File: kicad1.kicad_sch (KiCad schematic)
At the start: 44 parts

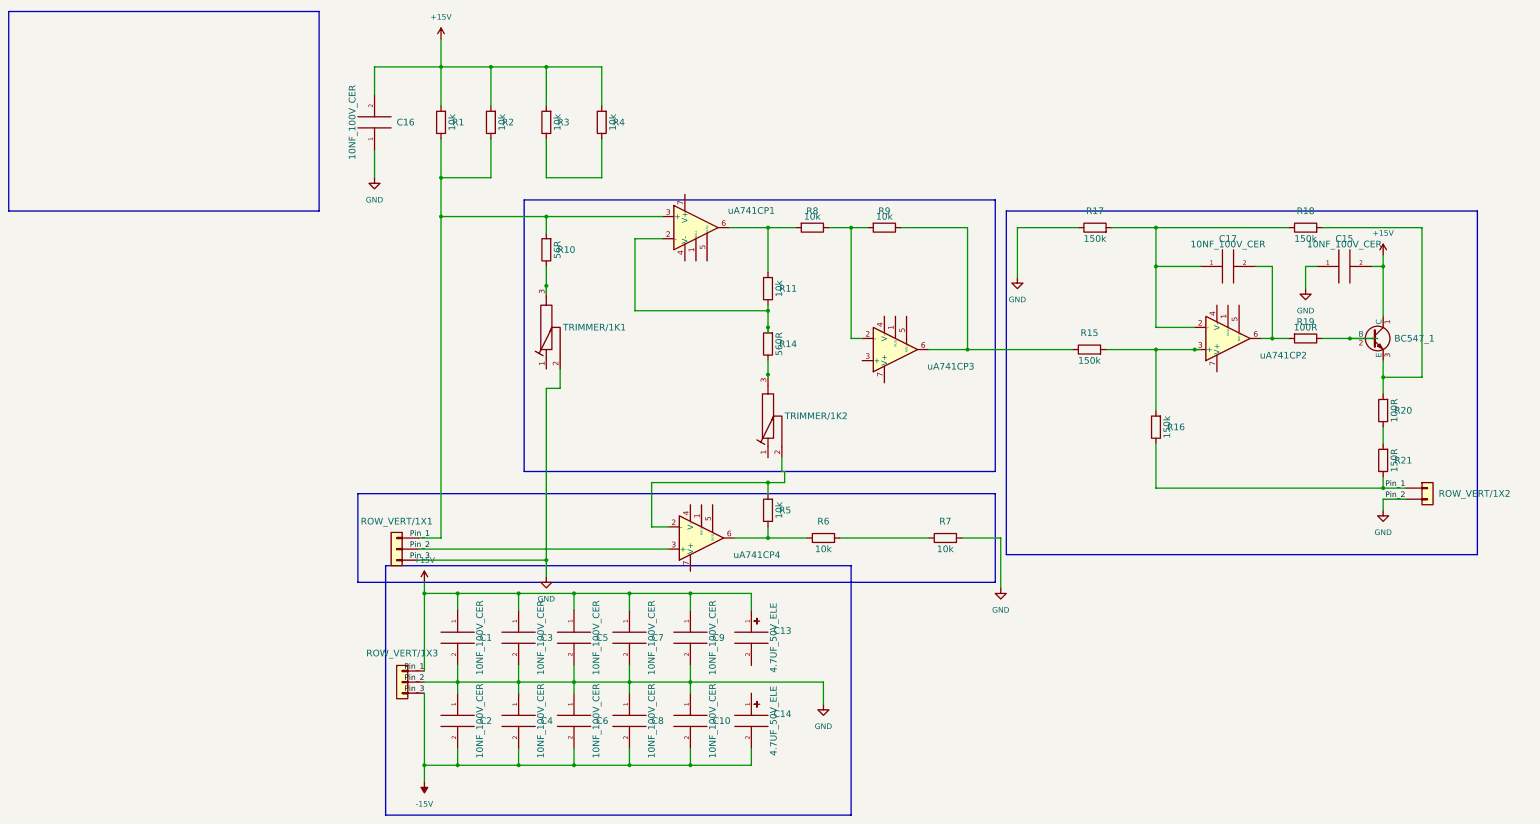
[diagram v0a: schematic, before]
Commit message: epätoivoinen versio ennen resettiä
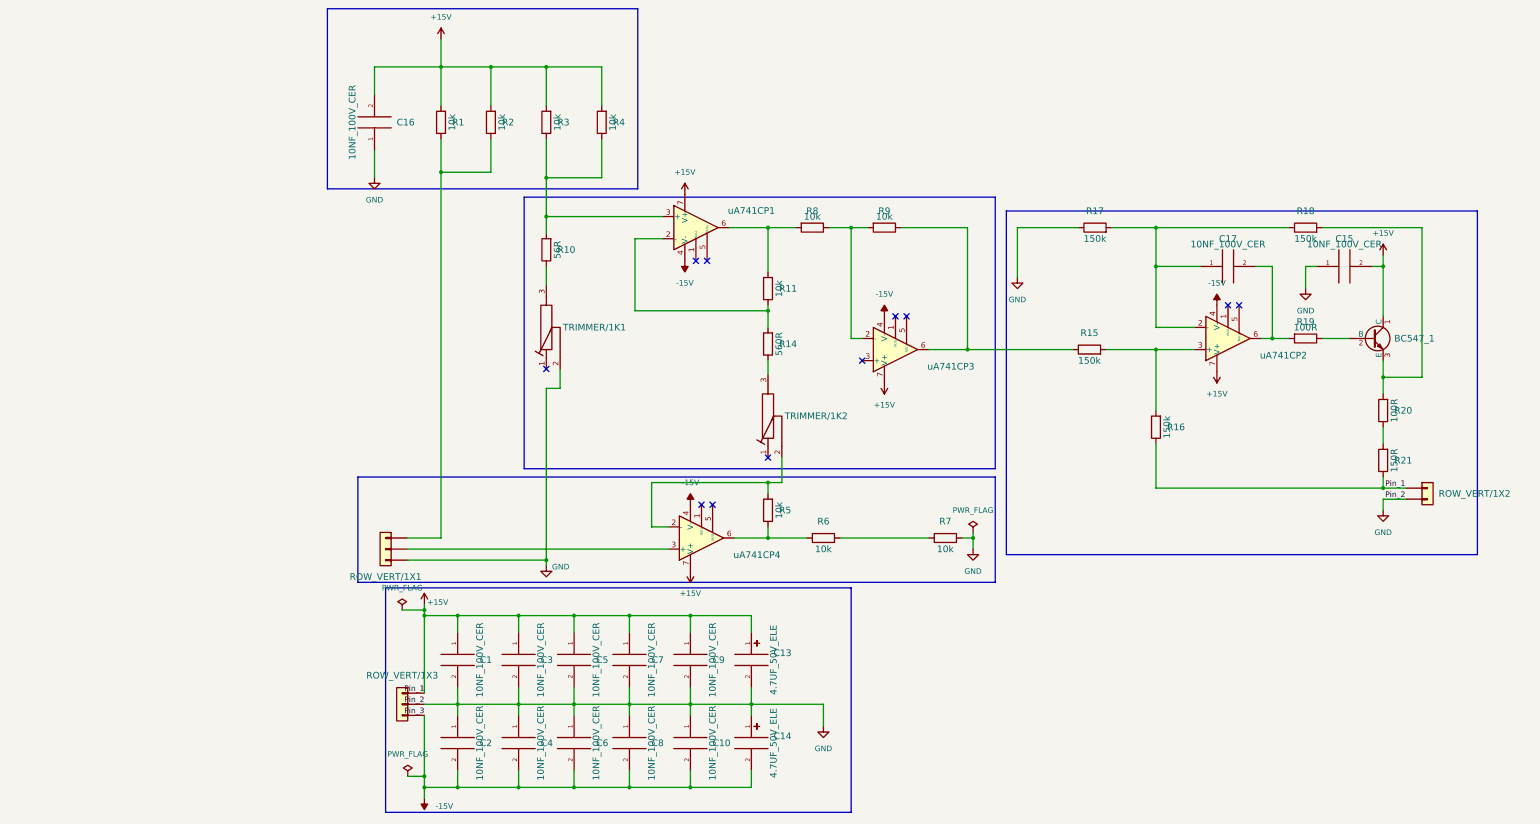
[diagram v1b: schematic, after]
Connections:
- net +15V: now also uA741CP1.7 (V+), uA741CP2.7 (V+), uA741CP3.7 (V+), uA741CP4.7 (V+); no longer R1.1, R10.2, R2.1, ROW_VERT/1X1.1 (Pin_1), uA741CP1.3 (+)
- net -15V: now also uA741CP1.4 (V-), uA741CP2.4 (V-), uA741CP3.4 (V-), uA741CP4.4 (V-); no longer C1.2, C10.1, C15.1, C16.1, C2.1, C3.2, C4.1, C5.2, C6.1, C7.2, C8.1, C9.2, R17.1, R7.2, ROW_VERT/1X1.2 (Pin_2), ROW_VERT/1X1.3 (Pin_3), ROW_VERT/1X2.2 (Pin_2), ROW_VERT/1X3.2 (Pin_2), TRIMMER/1K1.2, uA741CP4.3 (+)
- net at R3.1, R4.1: now also R10.2, uA741CP1.3 (+)
- net GND: now reaches C14.1
- net GND: now also C1.2, C10.1, C13.2, C15.1, C16.1, C2.1, C3.2, C4.1, C5.2, C6.1, C7.2, C8.1, C9.2, R17.1, R7.2, ROW_VERT/1X1.3 (Pin_3), ROW_VERT/1X2.2 (Pin_2), ROW_VERT/1X3.2 (Pin_2), TRIMMER/1K1.2
- new net: R1.1, R2.1, ROW_VERT/1X1.1 (Pin_1)
- new net: ROW_VERT/1X1.2 (Pin_2), uA741CP4.3 (+)
- no-connect marks 0 -> 11
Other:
- moved on the sheet: C1, C10, C13, C14, C2, C3, C4, C5, C6, C7, C8, C9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

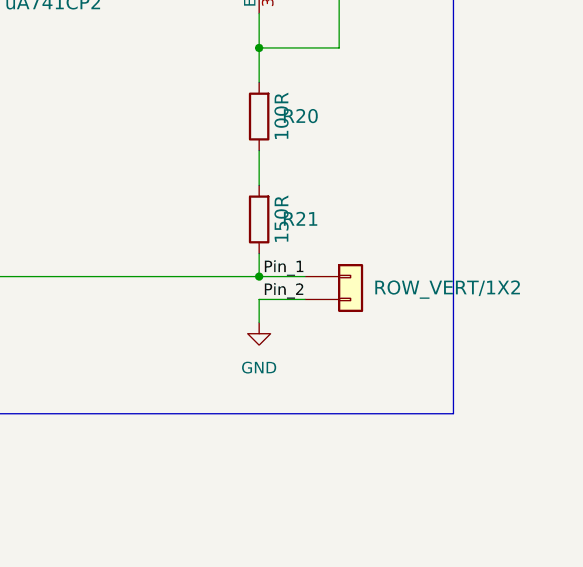
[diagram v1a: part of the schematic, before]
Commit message: done
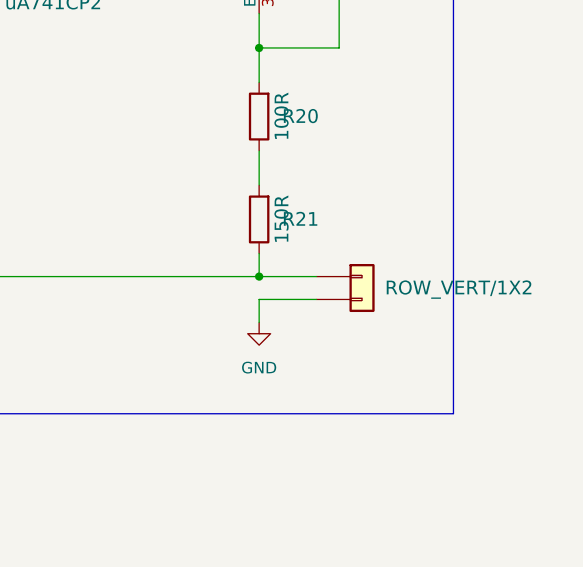
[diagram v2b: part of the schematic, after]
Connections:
- net +15V: no longer R16.1, R21.1, ROW_VERT/1X2.1 (Pin_1)
- new net: R16.1, R21.1, ROW_VERT/1X2.1 (Pin_1)
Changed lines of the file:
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@@
 	)
 	(junction
-		(at 88.9 172.72)
+		(at 261.62 123.19)
 		(diameter 0)
 		(color 0 0 0 0)
 	)
 	(junction
-		(at 261.62 123.19)
+		(at 88.9 172.72)
 		(diameter 0)
 		(color 0 0 0 0)
@@
 	(wire
 		(pts
-			(xy 266.7 123.19) (xy 261.62 123.19)
+			(xy 88.9 168.91) (xy 88.9 172.72)
 		)
 		(stroke
@@
 	(wire
 		(pts
-			(xy 88.9 168.91) (xy 88.9 172.72)
+			(xy 261.62 125.73) (xy 261.62 128.27)
 		)
 		(stroke
@@
 	(wire
 		(pts
-			(xy 261.62 125.73) (xy 261.62 128.27)
+			(xy 49.53 172.72) (xy 49.53 168.91)
 		)
 		(stroke
@@
 	(wire
 		(pts
-			(xy 49.53 172.72) (xy 49.53 168.91)
+			(xy 102.87 172.72) (xy 102.87 175.26)
 		)
 		(stroke
@@
 	(wire
 		(pts
-			(xy 102.87 172.72) (xy 102.87 175.26)
+			(xy 261.62 123.19) (xy 267.97 123.19)
 		)
 		(stroke
@@
 	(wire
 		(pts
-			(xy 266.7 125.73) (xy 261.62 125.73)
+			(xy 261.62 125.73) (xy 267.97 125.73)
 		)
 		(stroke
@@
 		)
 	)
-	(label "Pin_2"
-		(at 266.7 125.73 180)
-		(effects
-			(font
-				(size 1.27 1.27)
-			)
-			(justify right bottom)
-		)
-	)
 	(label "Pin_3"
 		(at 41.91 175.26 180)
@@
 		)
 	)
-	(label "Pin_1"
-		(at 266.7 123.19 180)
-		(effects
-			(font
-				(size 1.27 1.27)
-			)
-			(justify right bottom)
-		)
-	)
 	(symbol
 		(lib_id "VAMK_R:10k")
@@
 	)
 	(symbol
-		(lib_id "VAMK_CON:ROW_VERT_1X2")
-		(at 271.78 123.19 0)
-		(unit 1)
-		(exclude_from_sim no)
-		(in_bom yes)
-		(on_board yes)
-		(dnp no)
-		(fields_autoplaced yes)
-		(property "Reference" "ROW_VERT/1X2"
-			(at 274.32 124.4599 0)
-			(effects
-				(font
-					(size 1.524 1.524)
-				)
-				(justify left)
-			)
-		)
-		(property "Value" "ROW_VERT_1X2"
-			(at 287.02 120.65 0)
-			(effects
-				(font
-					(size 1.524 1.524)
-				)
-				(hide yes)
-			)
-		)
-		(property "Footprint" "VAMK_CON:ROW_VERT_1x2"
-			(at 287.02 123.19 0)
-			(effects
-				(font
-					(size 1.524 1.524)
-				)
-				(hide yes)
-			)
-		)
-		(property "Datasheet" "\"\""
-			(at 287.02 125.73 0)
-			(effects
-				(font
-					(size 1.524 1.524)
-				)
-				(hide yes)
-			)
-		)
-		(property "Description" "Plug, Vertical Row Header"
-			(at 271.78 123.19 0)
-			(effects
-				(font
-					(size 1.27 1.27)
-				)
-				(hide yes)
-			)
-		)
-		(property "Storing Location" "3.10.1.X"
-			(at 287.02 128.27 0)
-			(effects
-				(font
-					(size 1.524 1.524)
-				)
-				(hide yes)
-			)
-		)
-		(property "Order Number Elfa" "43-702-19"
-			(at 287.02 130.81 0)
-			(effects
-				(font
-					(size 1.524 1.524)
-				)
-				(hide yes)
-			)
-		)
-		(property "Order Numer Farnell" "329-1807"
-			(at 287.02 133.35 0)
-			(effects
-				(font
-					(size 1.524 1.524)
-				)
-				(hide yes)
-			)
-		)
-		(pin "1"
-		)
-		(pin "2"
-		)
-		(instances
-			(project ""
-				(path "/18748843-9013-4568-915a-7f405377b023"
-					(reference "ROW_VERT/1X2")
-					(unit 1)
-				)
-			)
-		)
-	)
-	(symbol
 		(lib_id "power:GND")
 		(at 167.64 137.16 0)
@@
 					(unit 1)
 				)
+			)
+		)
+	)
+	(symbol
+		(lib_id "VAMK_CON:ROW_VERT_1X2")
+		(at 273.05 123.19 0)
+		(unit 1)
+		(exclude_from_sim no)
+		(in_bom yes)
+		(on_board yes)
+		(dnp no)
+		(fields_autoplaced yes)
+		(property "Reference" "ROW_VERT/1X2"
+			(at 275.59 124.4599 0)
+			(effects
+				(font
+					(size 1.524 1.524)
+				)
+				(justify left)
+			)
+		)
+		(property "Value" "ROW_VERT_1X2"
+			(at 288.29 120.65 0)
+			(effects
+				(font
+					(size 1.524 1.524)
+				)
+				(hide yes)
+			)
+		)
+		(property "Footprint" "VAMK_CON:ROW_VERT_1x2"
+			(at 288.29 123.19 0)
+			(effects
+				(font
+					(size 1.524 1.524)
+				)
+				(hide yes)
+			)
+		)
+		(property "Datasheet" "\"\""
+			(at 288.29 125.73 0)
+			(effects
+				(font
+					(size 1.524 1.524)
+				)
+				(hide yes)
+			)
+		)
+		(property "Description" "Plug, Vertical Row Header"
+			(at 273.05 123.19 0)
+			(effects
+				(font
+					(size 1.27 1.27)
+				)
+				(hide yes)
+			)
+		)
+		(property "Storing Location" "3.10.1.X"
+			(at 288.29 128.27 0)
+			(effects
+				(font
+					(size 1.524 1.524)
+				)
+				(hide yes)
+			)
+		)
+		(property "Order Number Elfa" "43-702-19"
+			(at 288.29 130.81 0)
+			(effects
+				(font
+					(size 1.524 1.524)
+				)
+				(hide yes)
+			)
+		)
+		(property "Order Numer Farnell" "329-1807"
+			(at 288.29 133.35 0)
+			(effects
+				(font
+					(size 1.524 1.524)
+				)
+				(hide yes)
+			)
+		)
+		(pin "1"
+		)
+		(pin "2"
+		)
+		(instances
+			(project ""
+				(path "/18748843-9013-4568-915a-7f405377b023"
+					(reference "ROW_VERT/1X2")
+					(unit 1)
+				)
